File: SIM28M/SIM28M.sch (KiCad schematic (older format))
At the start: 25 parts, among them IC1 SIM28M, J1 Conn_01x05, J2 Conn_01x05, U2 AP7365-W-7

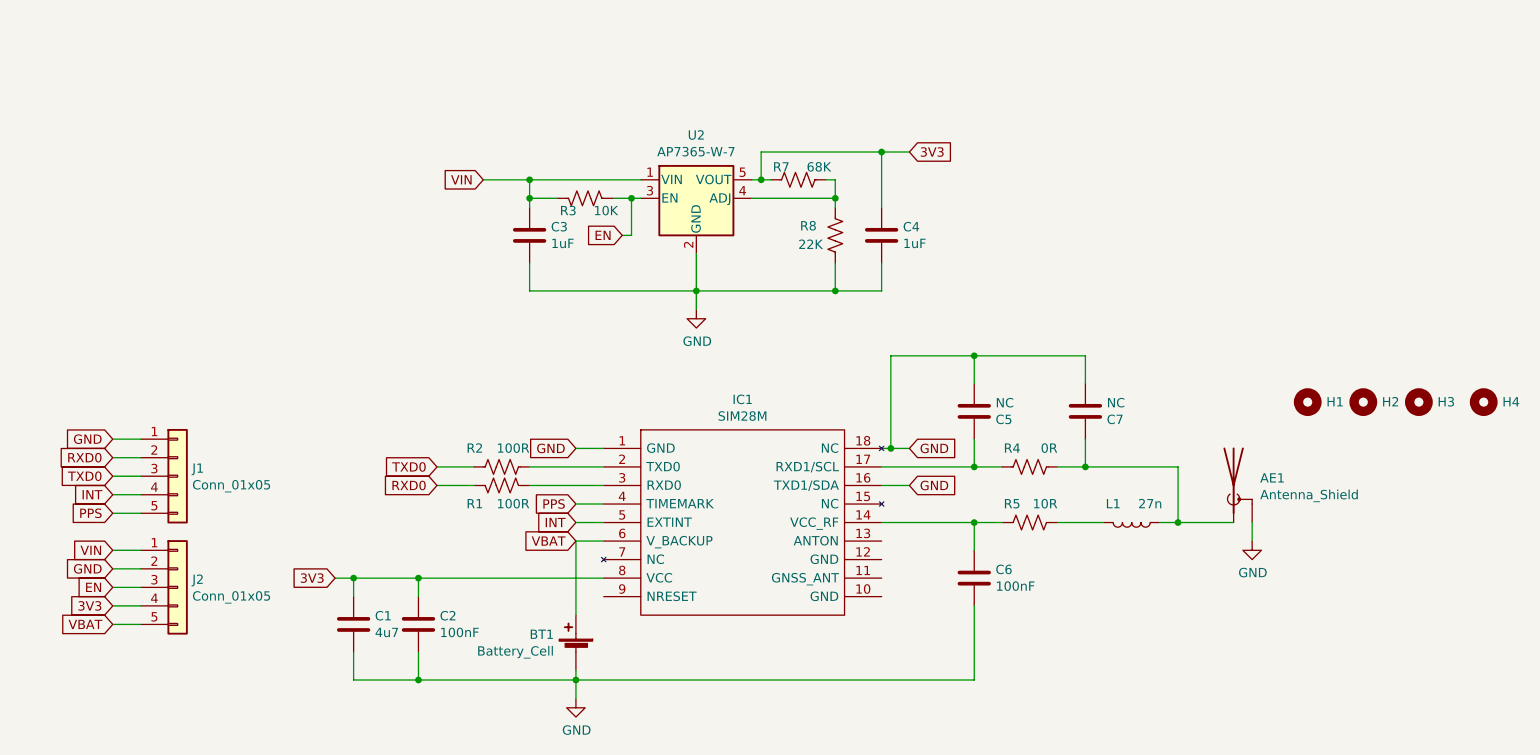
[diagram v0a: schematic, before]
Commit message: Layout Updated
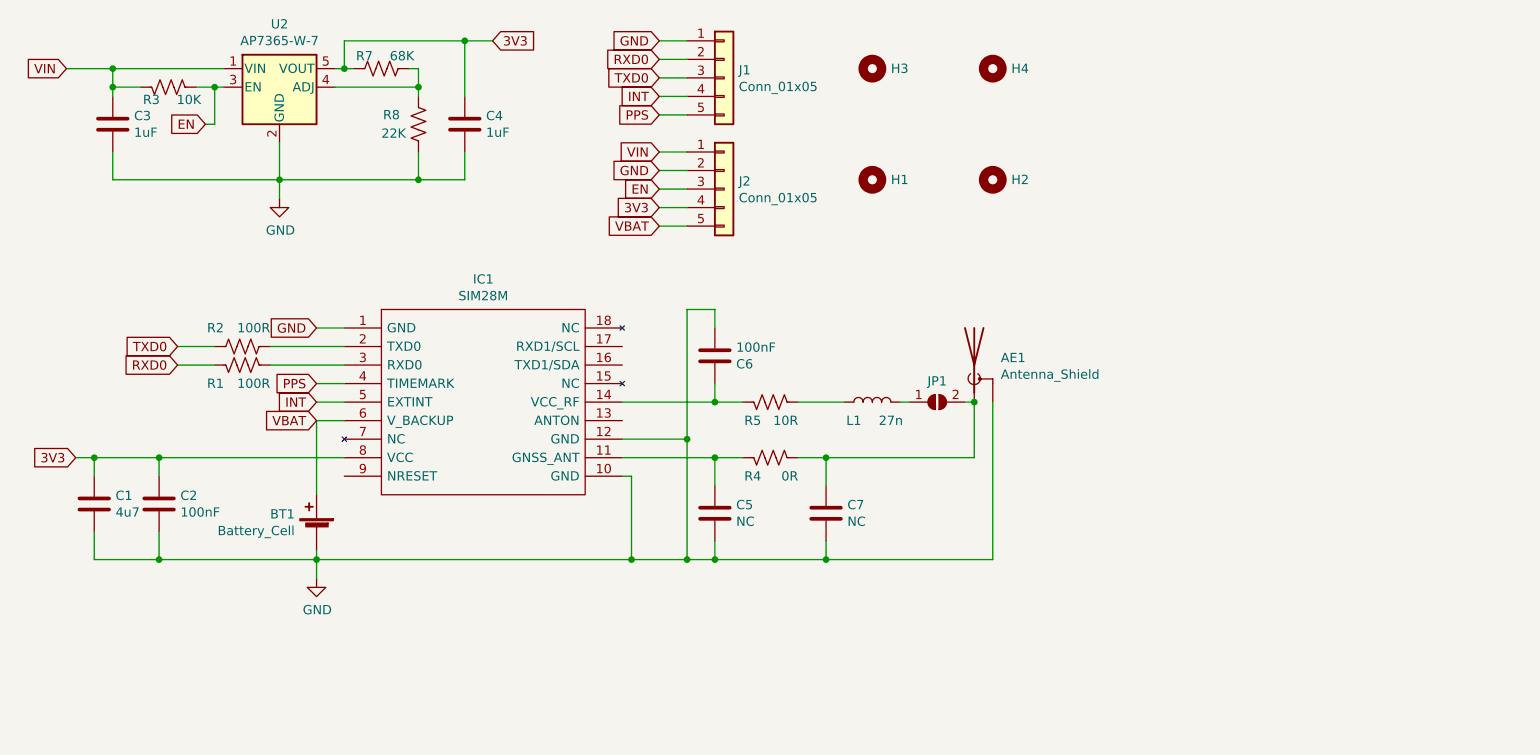
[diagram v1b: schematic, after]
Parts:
- added JP1: SolderJumper_2_Open, Jumper:SolderJumper-2_P1.3mm_Open_RoundedPad1.0x1.5mm, symbol Jumper:SolderJumper_2_Open
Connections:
- net GND: now also IC1.10 (GND), IC1.12 (GND); no longer IC1.16 (TXD1/SDA), IC1.18 (NC)
- net at IC1.11 (GNSS_ANT): now also C5.1, R4.1
- net at AE1.1 (A), C7.1, R4.2: now also JP1.2 (B); no longer L1.1
- new net: JP1.1 (A), L1.1
- now unconnected: IC1.17 (RXD1/SCL)
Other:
- moved on the sheet: AE1, BT1, C1, C2, C3, C4, C5, C6, C7, H1, H2, H3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
